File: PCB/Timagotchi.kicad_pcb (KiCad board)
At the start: 2 copper layers, 85 x 30 mm, 12 parts, among them J1 Conn_01x04, J2 Conn_01x02_Pin, SW1 SW_Omron_B3FS, SW2 SW_Omron_B3FS, SW3 SW_Omron_B3FS, U1 XIAO-ESP32-S3-Plus-SMD, U2 MAX98357A

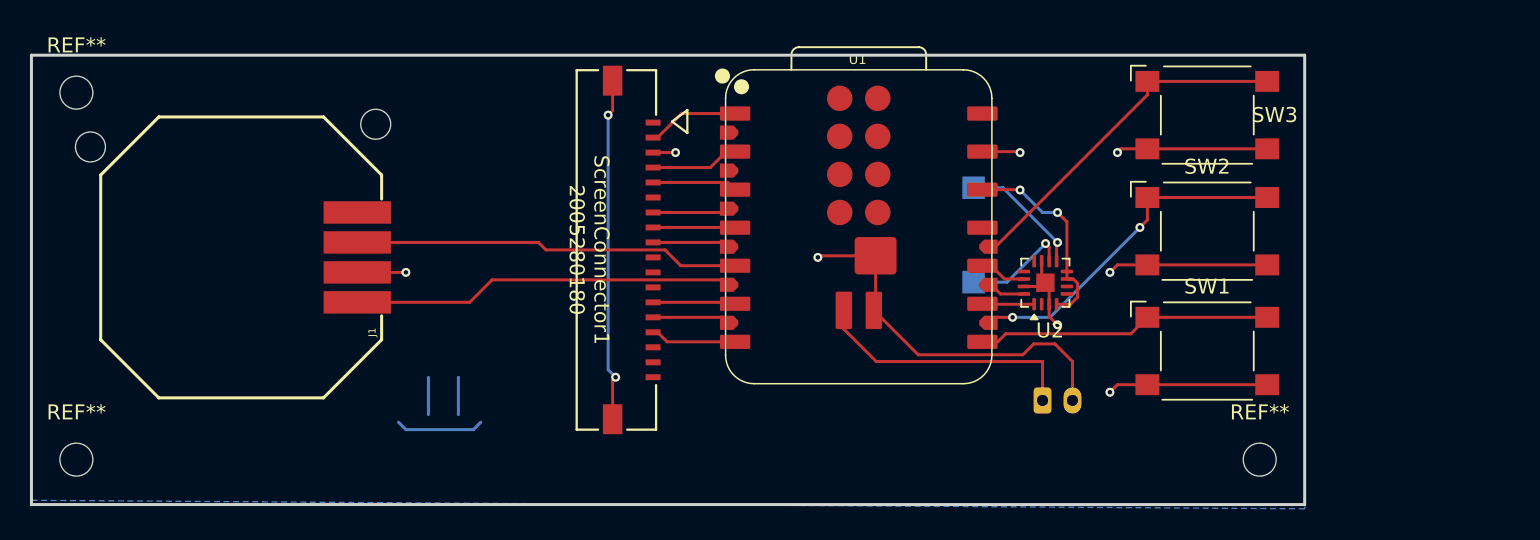
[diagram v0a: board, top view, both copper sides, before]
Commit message: PCB UHH delete later maybe
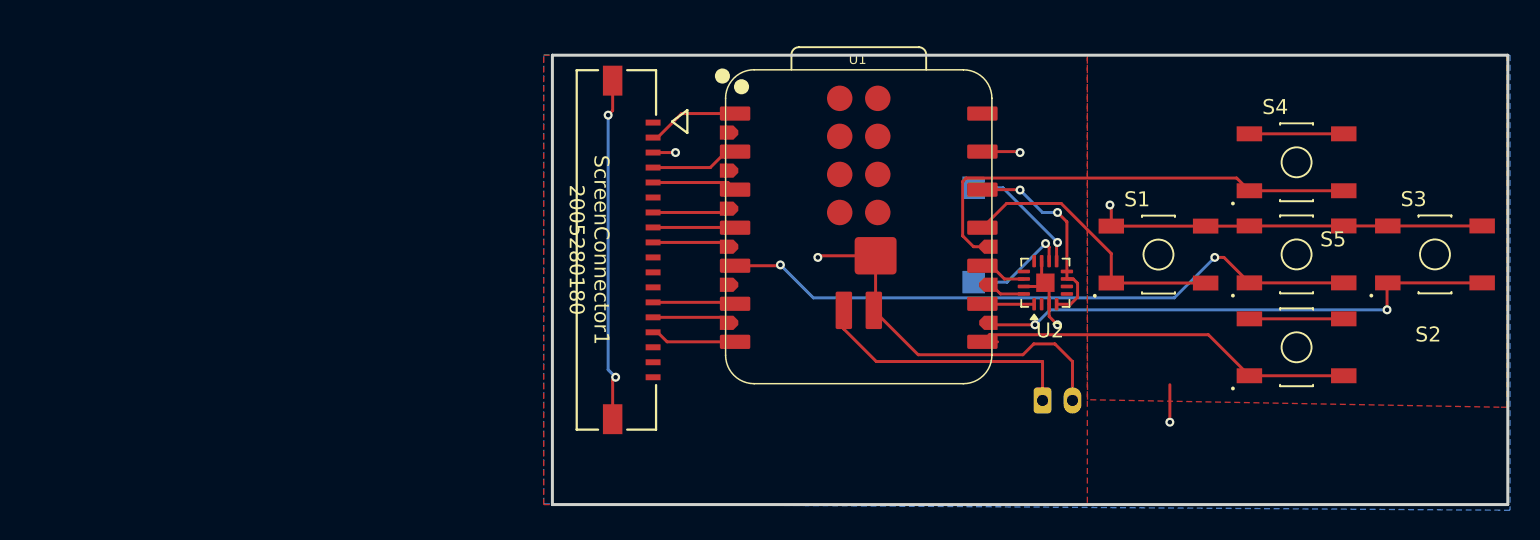
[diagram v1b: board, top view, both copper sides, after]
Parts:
- removed J1: Conn_01x04, Library:JOYSTICK-PSP1000
- removed REF** (x3): MountingHole_2.2mm_M2, MountingHole:MountingHole_2.2mm_M2
- removed SW1, SW2, SW3: SW_Omron_B3FS, Button_Switch_SMD:SW_SPST_Omron_B3FS-100xP
- added S1: TL3342F160QG, Switch Footprints:SW_TL3342F160QG, F.Cu at (204.2, 51.8)
- added S2: TL3342F160QG, Switch Footprints:SW_TL3342F160QG, F.Cu at (213.5, 58.0)
- added S3: TL3342F160QG, Switch Footprints:SW_TL3342F160QG, F.Cu at (222.7, 51.8)
- added S4: TL3342F160QG, Switch Footprints:SW_TL3342F160QG, F.Cu at (213.5, 45.6)
- added S5: TL3342F160QG, Switch Footprints:SW_TL3342F160QG, F.Cu at (213.5, 51.8)
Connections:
- U1 pad 11: unconnected-(U1-GPIO9_A10_D10_MOSI-Pad11) -> /SW1
- U1 pad 19: /HPOS -> unconnected-(U1-GPIO42_PDM_CLK_TX1-Pad19)
- U1 pad 21: /SW2 -> /SW3
- U1 pad 23: /SW3 -> /SW4
- U1 pad 5: /VPOS -> /SW5
- U1 pad 8: /SW1 -> /SW2
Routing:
- net /SW5: track 0.00 -> 43.4 mm, vias 0 -> 2
- net /SW4: track 0.00 -> 32.0 mm
- net /VPOS: track 25.9 -> 0.00 mm
- net /HPOS: track 25.6 -> 0.00 mm
- net /SW3: track 23.7 -> 35.7 mm, vias 0 -> 2
- net (no net): track 10.9 -> 2.50 mm, vias 0 -> 1
- net GND: track 93.5 -> 97.6 mm, vias 10 -> 7
- net /SW2: track 23.0 -> 26.5 mm, vias 2 -> 0
- net /SW1: track 19.7 -> 18.9 mm
- added copper zone on F.Cu, net GND
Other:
- board size 85 x 30 mm -> 63.8 x 30 mm

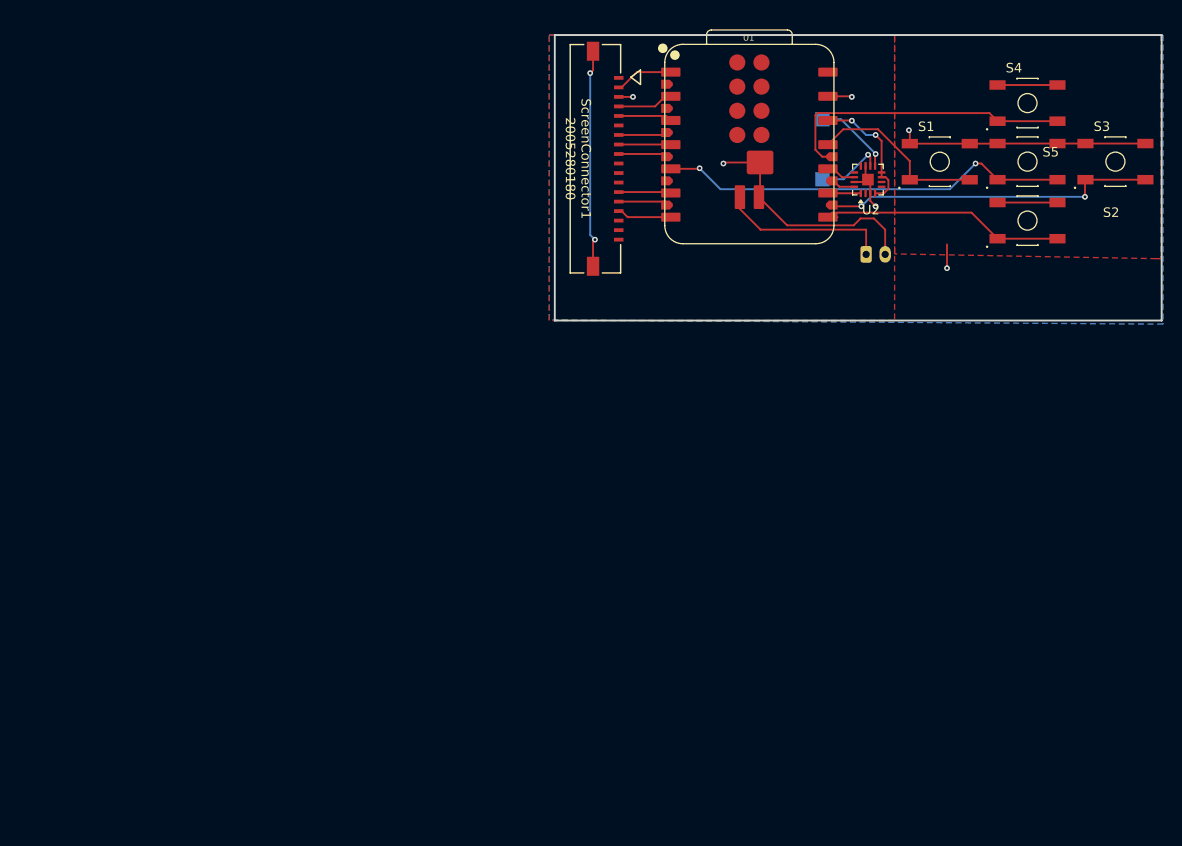
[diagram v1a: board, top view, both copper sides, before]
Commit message: lots of stuff
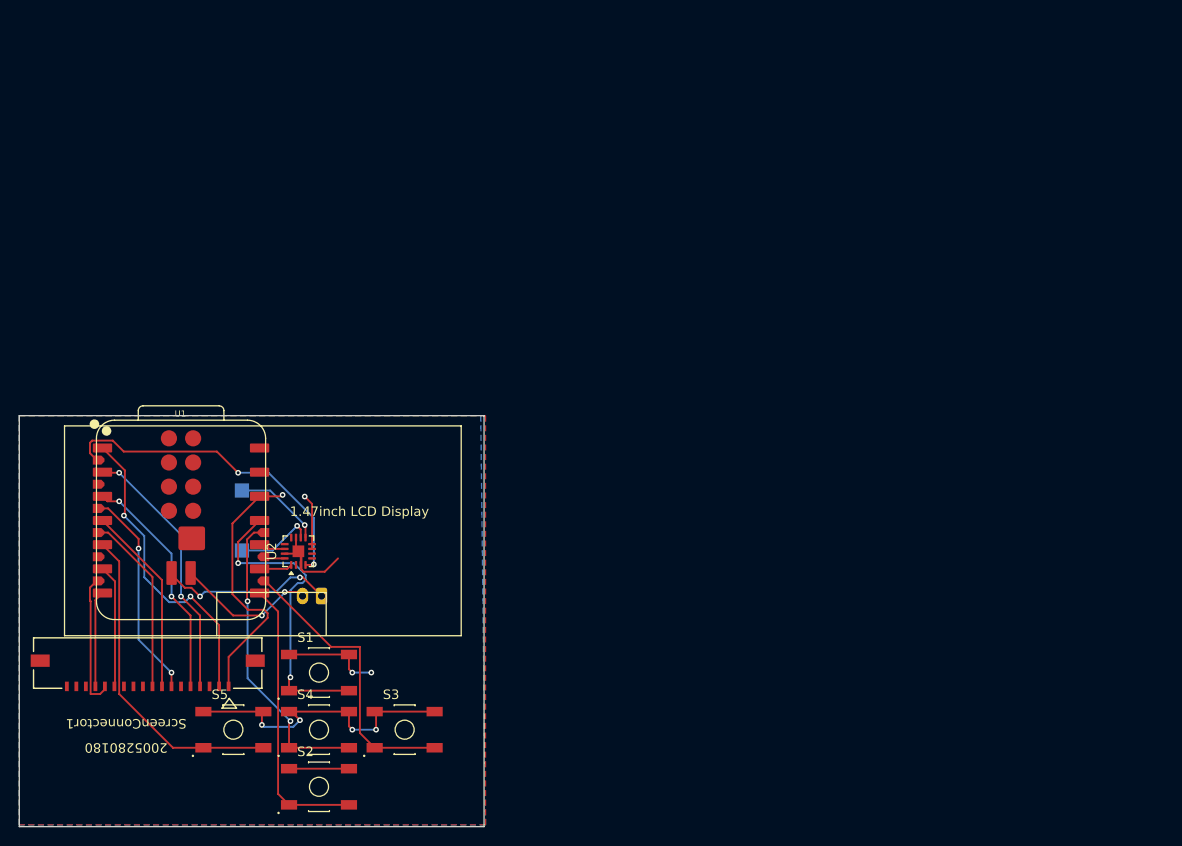
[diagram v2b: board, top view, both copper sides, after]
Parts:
- added 1.47inch LCD Display: 1.47inch LCD Display, Library:1.47inch LCD Display, F.Cu at (112.3, 79.6)
- moved S5 102.6 mm to (130.0, 111.5)
- moved S4 99.4 mm to (139.0, 111.5)
- moved S3 95.6 mm to (148.0, 111.5)
- moved S2 95.3 mm to (139.0, 117.5)
- moved S1 84.5 mm to (139.0, 105.5)
- moved LS1 72.4 mm to (124.5, 89.5)
- moved U1 71.6 mm to (124.5, 89.5)
- moved U2 71.5 mm to (136.8, 92.8)
- moved ScreenConnector1 70.9 mm to (121.0, 104.5), turned to 180 degrees
- moved J2 67.6 mm to (139.3, 97.5), turned to 180 degrees
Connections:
- U1 pad 15: unconnected-(U1-GPIO38_DVP_VSYNC_I2S_SD-Pad15) -> /SD_MODE
- U2 pad 4: +3.3V -> /SD_MODE
- U2 pad 7: +3.3V -> Net-(C1-Pad2)
- U2 pad 8: +3.3V -> Net-(C1-Pad2)
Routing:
- net /SD_MODE: track 0.00 -> 35.1 mm, vias 0 -> 2
- net /LCD_BL: track 6.14 -> 32.4 mm, vias 0 -> 2
- net GND: track 97.6 -> 75.5 mm, vias 7 -> 8
- net /SCLK: track 5.92 -> 27.8 mm, vias 0 -> 2
- net /MOSI: track 5.67 -> 24.5 mm, vias 0 -> 2
- net /TP_INT: track 5.18 -> 22.5 mm, vias 0 -> 2
- net /LCD_RST: track 5.48 -> 20.0 mm
- net +3.3V: track 13.7 -> 27.9 mm, vias 2 -> 1
- net /LCD_CS: track 5.19 -> 19.1 mm
- net /SW1: track 18.9 -> 32.5 mm, vias 0 -> 2
- net /SW5: track 43.4 -> 33.9 mm, vias 2 -> 0
- net /TP_SDA: track 5.23 -> 14.4 mm
- net /TP_SCL: track 5.51 -> 12.9 mm
- net Net-(C1-Pad2): track 0.00 -> 5.82 mm, vias 0 -> 1
- net /SW3: track 35.7 -> 30.6 mm, vias 2 -> 0
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- added copper zone on B.Cu, net +3.3V
- removed copper zone on F.Cu, net +3.3V
- removed copper zone on B.Cu, net GND
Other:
- board size 63.8 x 30 mm -> 48.8 x 43.2 mm
